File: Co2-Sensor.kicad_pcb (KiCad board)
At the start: 2 copper layers, 45 x 65 mm, 85 parts, among them J1 OLED, J2 SCD30, J3 LED, J4 Power, J5 USB_C_Receptacle_USB2.0, J6 LED, J7 SPS30, J8 I2C, Q1 S8050, Q2 S8050, Q3 2N7002, Q4 2N7002, SW1 USER1, SW2 USER2, SW3 USER3, SW4 PROGRAM, U1 ESP32-WROOM-32D, U2 AMS1117-3.3, U3 CP2102, U4 BMP280, U5 74LVC1G02

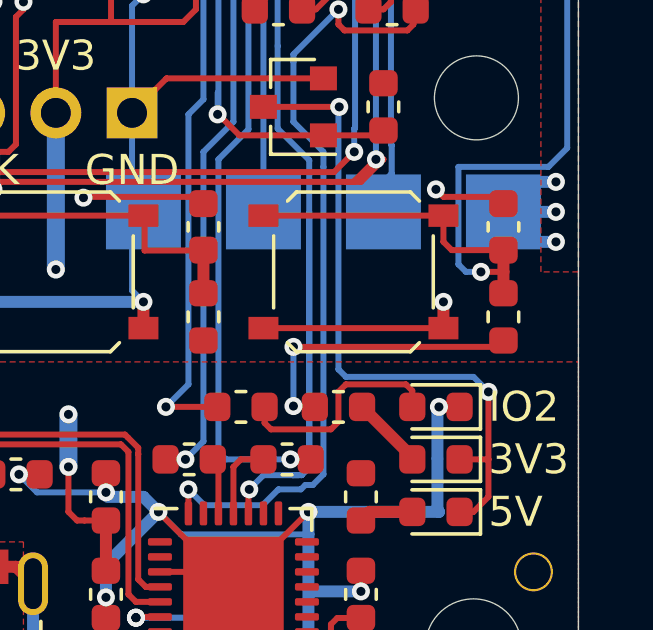
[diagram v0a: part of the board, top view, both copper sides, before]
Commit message: Revision 2
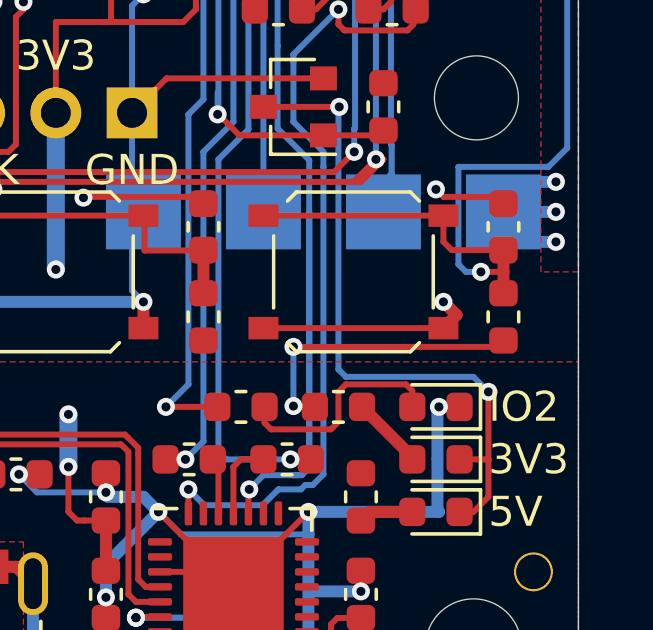
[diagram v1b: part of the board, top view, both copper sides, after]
